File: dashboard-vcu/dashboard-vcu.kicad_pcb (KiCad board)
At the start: 2 copper layers, 64.8 x 73.7 mm, 26 parts, among them IC2 TIP102, IC3 TIP102, J1 39300140, U1 Pico, U2 MCP2515-xSO, U3 SN65HVD230

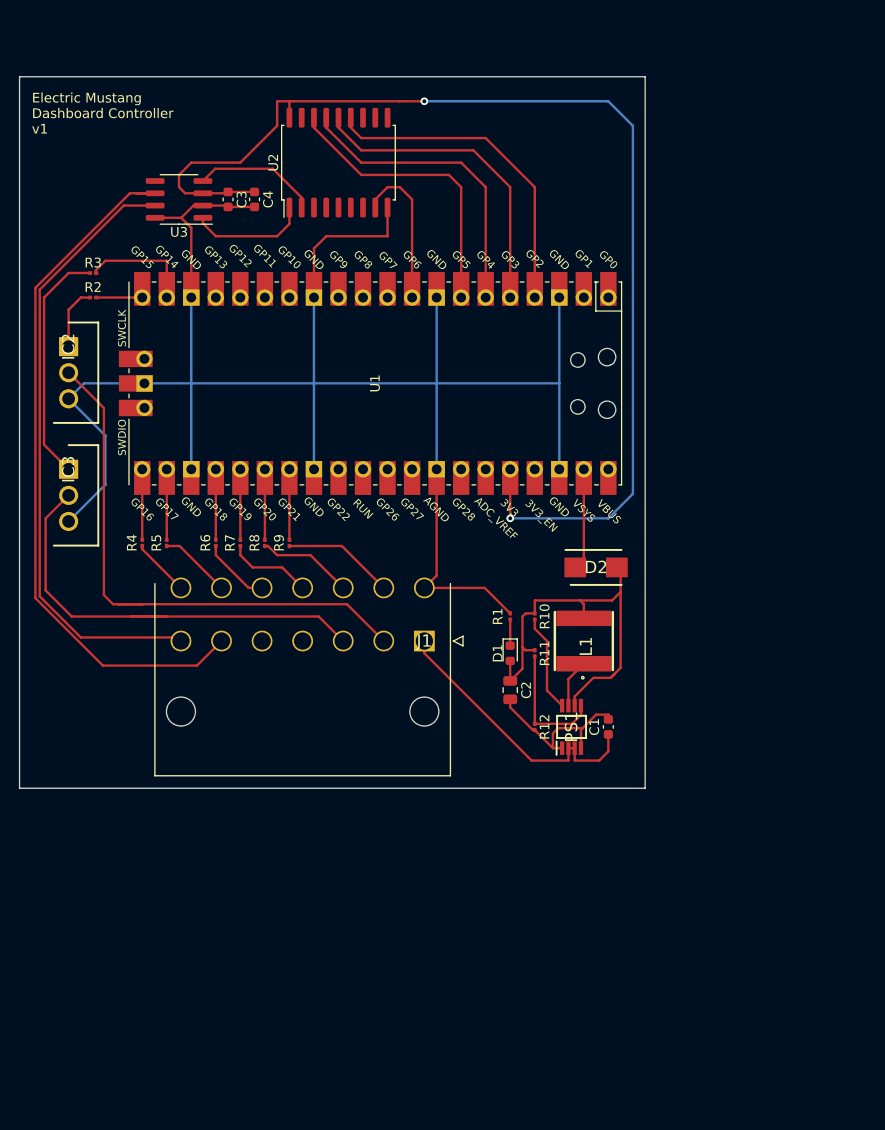
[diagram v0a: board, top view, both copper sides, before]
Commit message: Dashboard vcu update
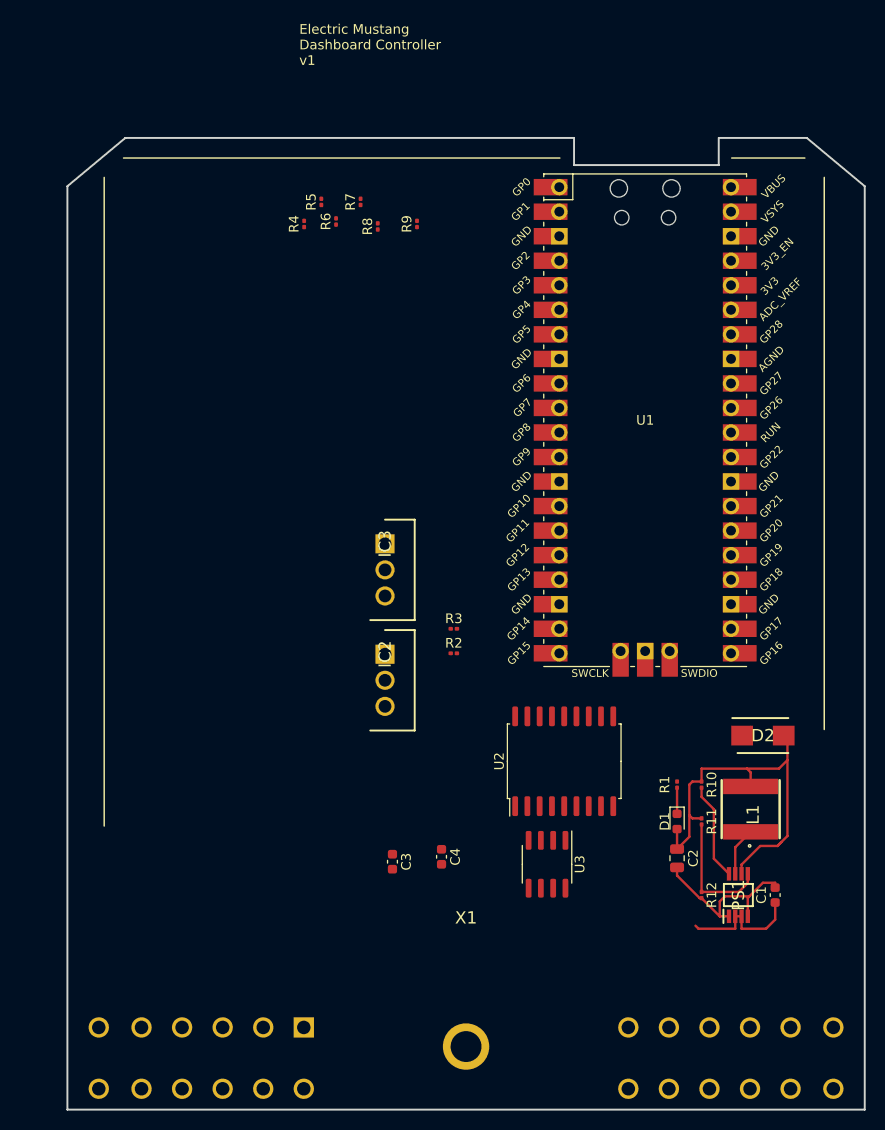
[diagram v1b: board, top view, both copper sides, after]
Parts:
- removed J1: 39300140, Connector:39300140
- added X1: ATM13-12PB-12PC-BM03, Connector:ATM1312PB12PCBM03, F.Cu at (127.2, 139.1)
- moved U3 78.7 mm to (152.4, 122.2), turned to -90 degrees
- moved C4 70.8 mm to (141.5, 121.4)
- moved C3 70.6 mm to (136.4, 121.9)
- moved U2 66.2 mm to (154.2, 111.5)
- moved R2 52.4 mm to (142.7, 100.3)
- moved R3 52.4 mm to (142.7, 97.8)
- moved IC2 45.7 mm to (135.6, 100.4)
- moved R5 38.8 mm to (129.0, 53.6)
- moved R7 37.4 mm to (133.1, 53.6)
- moved R4 37.0 mm to (127.3, 55.9)
- moved R9 35.6 mm to (138.9, 55.9)
- moved R6 35.5 mm to (130.6, 55.6)
- moved R8 34.8 mm to (134.9, 56.1)
- moved IC3 33.7 mm to (135.6, 89.0)
- moved U1 28.2 mm to (162.6, 76.2), turned to 0 degrees
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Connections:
- C1 pad 2: Net-(C1-Pad2) -> GND
- C2 pad 2: Net-(C1-Pad2) -> GND
- PS1 pad 1: Net-(C1-Pad2) -> GND
- PS1 pad 4: Net-(C1-Pad2) -> GND
- R12 pad 2: Net-(C1-Pad2) -> GND
- U1 pad 1: Net-(U1-Pad1) -> unconnected-(U1-Pad1)
- U1 pad 10: Net-(U1-Pad10) -> unconnected-(U1-Pad10)
- U1 pad 11: Net-(U1-Pad11) -> unconnected-(U1-Pad11)
- U1 pad 12: Net-(U1-Pad12) -> unconnected-(U1-Pad12)
- U1 pad 2: Net-(U1-Pad2) -> unconnected-(U1-Pad2)
- U1 pad 29: Net-(U1-Pad29) -> unconnected-(U1-Pad29)
- U1 pad 30: Net-(U1-Pad30) -> unconnected-(U1-Pad30)
- U1 pad 31: Net-(U1-Pad31) -> unconnected-(U1-Pad31)
- U1 pad 32: Net-(U1-Pad32) -> unconnected-(U1-Pad32)
- U1 pad 34: Net-(U1-Pad34) -> unconnected-(U1-Pad34)
- U1 pad 35: Net-(U1-Pad35) -> unconnected-(U1-Pad35)
- U1 pad 37: Net-(U1-Pad37) -> unconnected-(U1-Pad37)
- U1 pad 40: Net-(U1-Pad40) -> unconnected-(U1-Pad40)
- U1 pad 41: Net-(U1-Pad41) -> unconnected-(U1-Pad41)
- U1 pad 43: Net-(U1-Pad43) -> unconnected-(U1-Pad43)
- U2 pad 10: Net-(U2-Pad10) -> unconnected-(U2-Pad10)
- U2 pad 11: Net-(U2-Pad11) -> unconnected-(U2-Pad11)
- U2 pad 12: Net-(U2-Pad12) -> unconnected-(U2-Pad12)
- U2 pad 17: Net-(U2-Pad17) -> unconnected-(U2-Pad17)
- U2 pad 3: Net-(U2-Pad3) -> unconnected-(U2-Pad3)
- U2 pad 4: Net-(U2-Pad4) -> unconnected-(U2-Pad4)
- U2 pad 5: Net-(U2-Pad5) -> unconnected-(U2-Pad5)
- U2 pad 6: Net-(U2-Pad6) -> unconnected-(U2-Pad6)
- U2 pad 7: Net-(U2-Pad7) -> unconnected-(U2-Pad7)
- U3 pad 5: Net-(U3-Pad5) -> unconnected-(U3-Pad5)
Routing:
- net GND: track 197.0 -> 18.7 mm
- net 3V: track 120.7 -> 0.00 mm, vias 2 -> 0
- net CAN_L: track 73.8 -> 0.00 mm
- net CAN_H: track 63.8 -> 0.00 mm
- net FUEL_GAUGE: track 58.0 -> 0.00 mm
- net TEMP_GAUGE: track 47.5 -> 0.00 mm
- net SPI0_CLK: track 34.1 -> 0.00 mm
- net SPI0_TX: track 32.8 -> 0.00 mm
- net SPI0_RX: track 31.5 -> 0.00 mm
- net SPI0_CS: track 30.2 -> 0.00 mm
- net Net-(IC3-Pad1): track 24.6 -> 0.00 mm
- net Net-(C1-Pad2): track 18.7 -> 0.00 mm
- net 12V: track 29.6 -> 13.1 mm
- net 8MHz: track 15.9 -> 0.00 mm
- net PWM3: track 14.2 -> 0.00 mm
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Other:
- board size 64.8 x 73.7 mm -> 82.6 x 100.6 mm
